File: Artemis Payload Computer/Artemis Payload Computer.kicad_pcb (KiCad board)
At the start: 2 copper layers, 13 parts, among them J1 Screw_Terminal_01x02, J2 Screw_Terminal_01x02, J601 Connector_Screw_Terminal_01x02, U1 HX711, U2 Teensy3.2, U401 ICM-20948, U501 BMP280, U601 MIC39100-5.0WS, U701 MicroSD_Breakout_Sparkfun

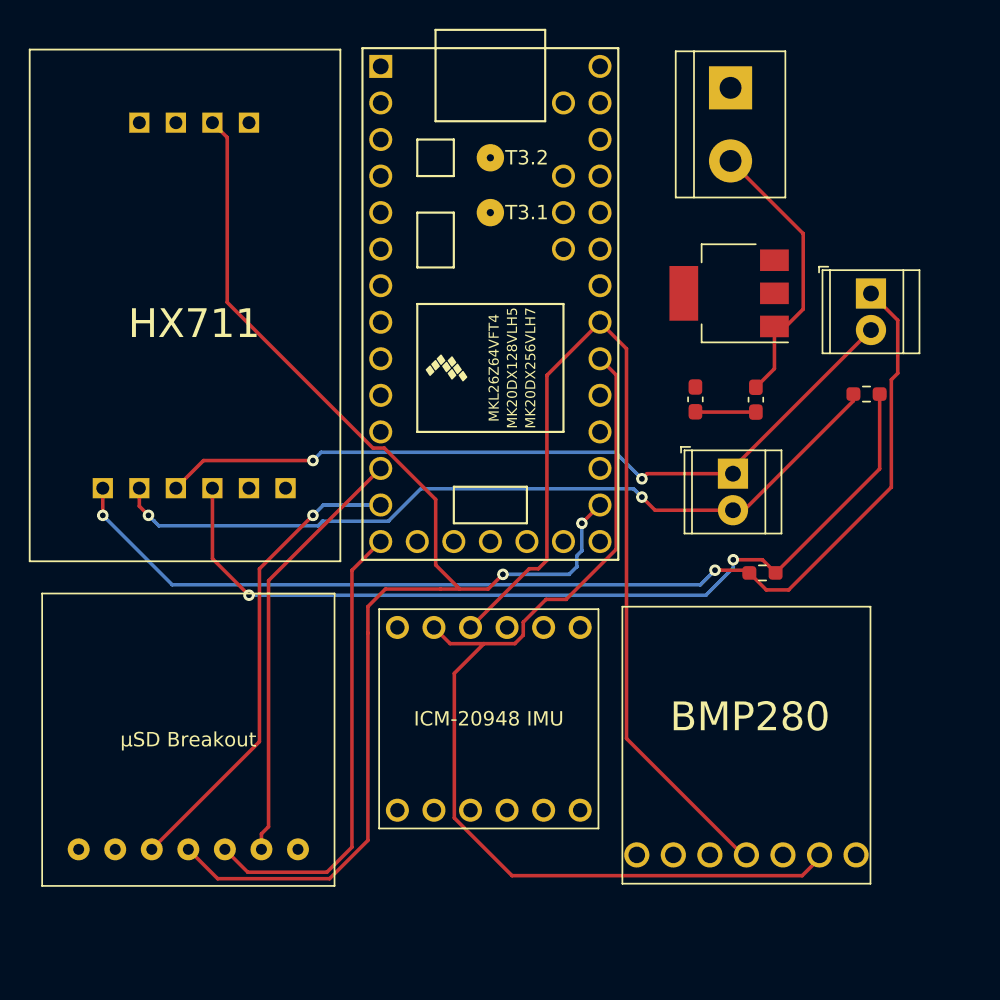
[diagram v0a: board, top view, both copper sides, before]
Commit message: ready for review
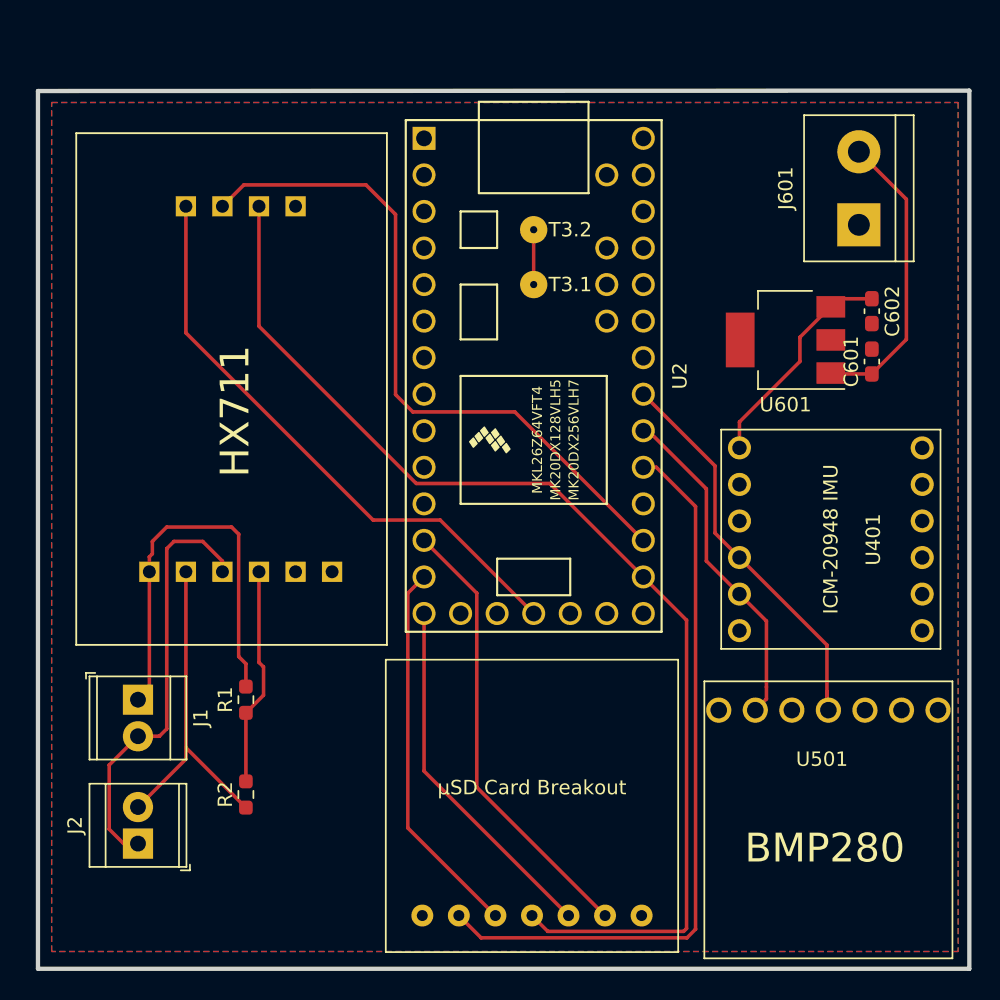
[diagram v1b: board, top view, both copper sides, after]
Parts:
- moved J1 58.2 mm to (125.0, 72.5)
- moved R2 51.3 mm to (132.5, 79.1), turned to 90 degrees
- moved J2 48.7 mm to (125.0, 82.5), turned to 90 degrees
- moved R1 37.0 mm to (132.5, 72.5), turned to 90 degrees
- moved U401 34.6 mm to (179.5, 55.0), turned to 270 degrees
- moved U701 24.3 mm to (160.0, 87.5)
- moved U501 23.2 mm to (180.6, 73.2), turned to 180 degrees
- moved C602 13.7 mm to (176.0, 45.5)
- moved J601 13.0 mm to (175.1, 39.5), turned to 90 degrees
- moved C601 8.48 mm to (176.0, 49.0), turned to 90 degrees
- moved U1 6.65 mm to (155.0, 72.5)
- moved U2 5.84 mm to (152.5, 50.0)
- moved U601 5.09 mm to (170.0, 47.5)
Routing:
- net /CD: track 0.00 -> 51.5 mm
- net Net-(J1-Pad1): track 77.1 -> 28.8 mm, vias 2 -> 0
- net /DT: track 0.00 -> 47.4 mm
- net /SDA0: track 70.6 -> 23.5 mm
- net Net-(R1-Pad1): track 62.2 -> 15.2 mm, vias 2 -> 0
- net /SCL0: track 66.8 -> 27.8 mm
- net GND: track 4.21 -> 41.0 mm
- net Net-(J2-Pad2): track 56.7 -> 23.6 mm, vias 2 -> 0
- net Net-(J1-Pad2): track 54.8 -> 29.8 mm, vias 2 -> 0
- net +5V: track 0.00 -> 15.5 mm
- net /SCK: track 91.3 -> 79.2 mm, vias 2 -> 0
- net /DI: track 32.3 -> 25.1 mm
- net /DO: track 32.9 -> 26.5 mm, vias 1 -> 0
- net Net-(U2-Pad52): track 0.00 -> 3.81 mm
- net /CS: track 29.9 -> 31.3 mm
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- added copper zone on B.Cu, net +5V
- added copper zone on F.Cu, net GND
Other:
- board outline added: 64.7 x 61 mm
